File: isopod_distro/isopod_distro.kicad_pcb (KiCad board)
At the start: 4 copper layers, 65 x 56.5 mm, 62 parts, among them J1 CHG_IN, J10 IN 1, J11 IN 2, J12 IN 3, J13 IN 4, J14 IN 5, J15 IN 6, J16 BATT, J17 OUT 7, J18 OUT 8, J19 OUT 9, J2 OUT 1, J20 OUT 10, J21 OUT 11, J22 OUT 12, J23 IN 7, J24 IN 8, J25 IN 9, J26 IN 10, J27 IN 11, J28 IN 12, J29 BAL, J3 OUT 2, J30 Raspberry_Pi_2_3, J4 OUT 3, J5 OUT 4, J6 OUT 5, J7 OUT 6, J8 DCDC, Q1 IRLR6225TRPBF, Q2 BSS138, Q3 BSS138, U1 MAX17205, U2 UPU-MAX-M8C, U3 adafruit_tdk_icm-20948

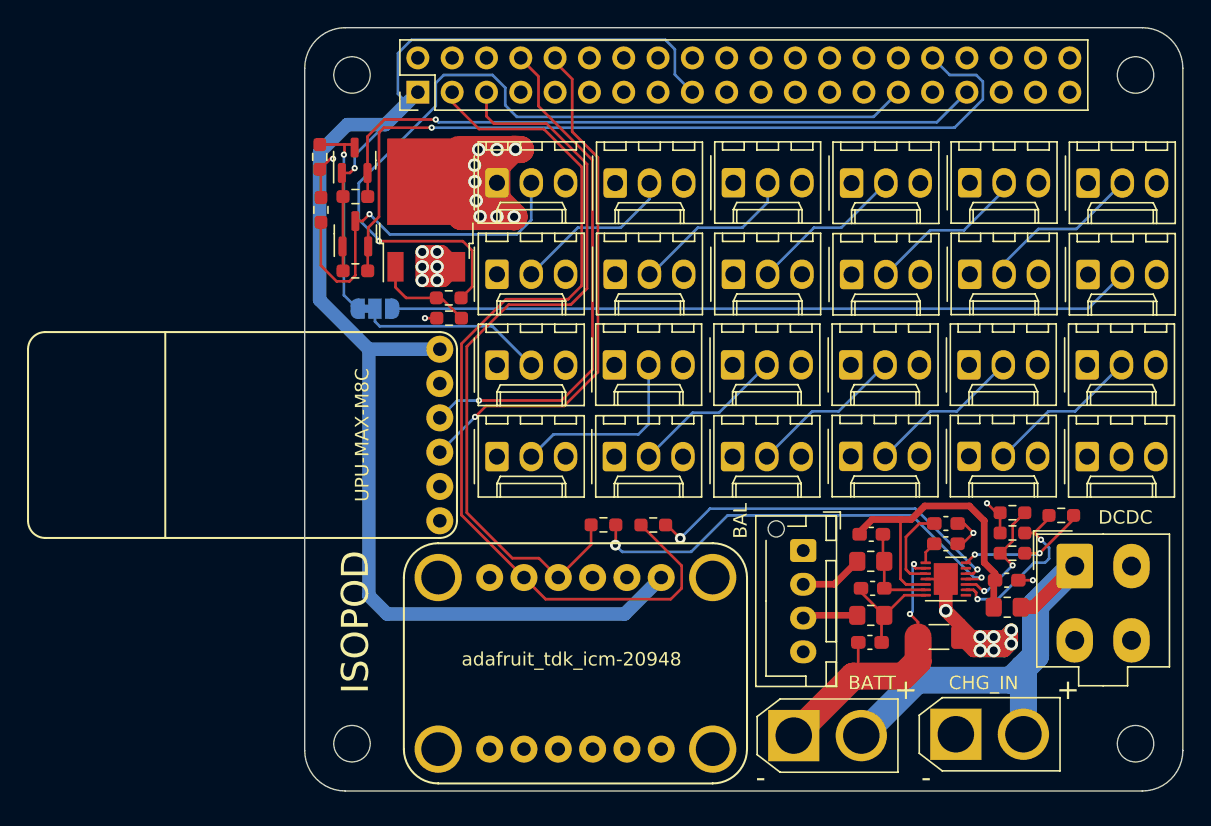
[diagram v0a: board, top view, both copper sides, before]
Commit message: DRC fixes/exclusions
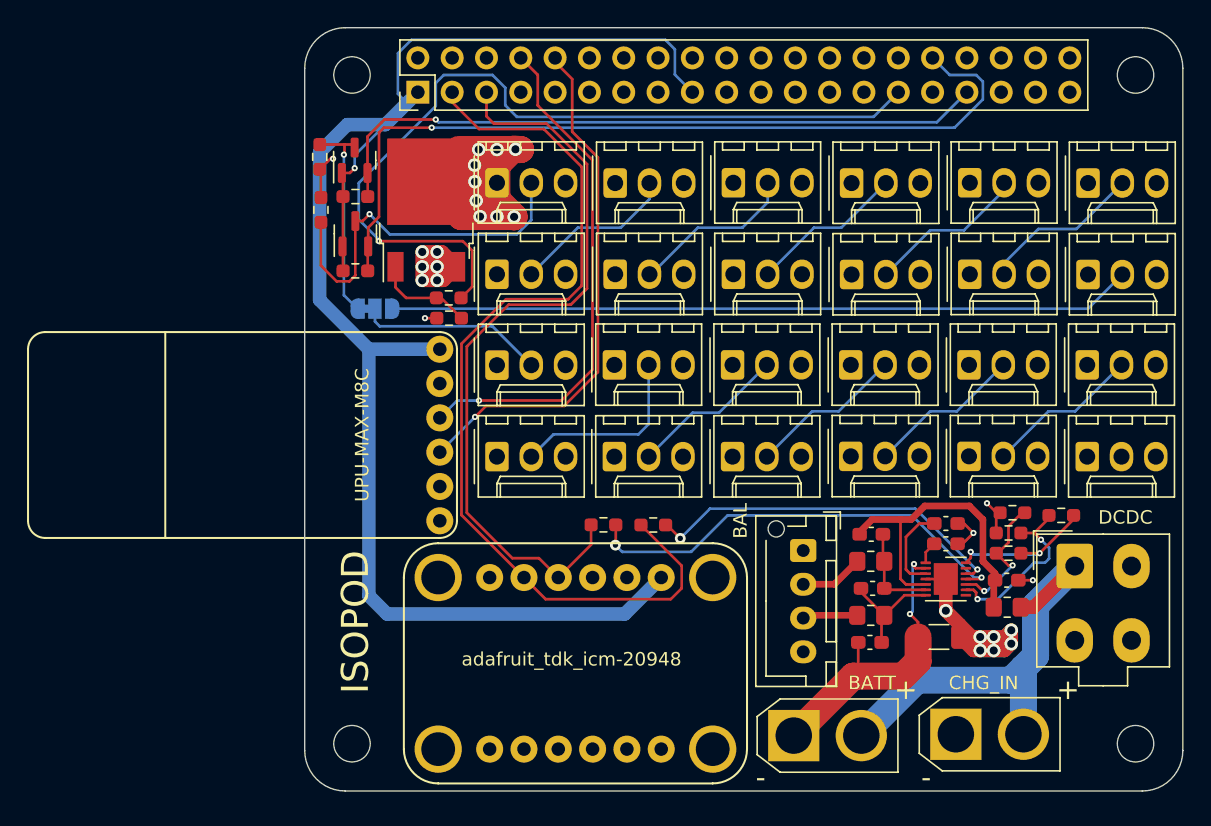
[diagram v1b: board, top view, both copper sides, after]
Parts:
- moved R14 0.29 mm to (202.1, 138.9)
- moved R15 0.29 mm to (202.1, 137.4)
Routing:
- net /GPS_RXD: track 38.8 -> 38.0 mm
- net Net-(R13-Pad1): track 10.7 -> 11.4 mm
